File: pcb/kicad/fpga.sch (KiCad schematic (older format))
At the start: 15 parts, among them U4 XC3S400-PQ208

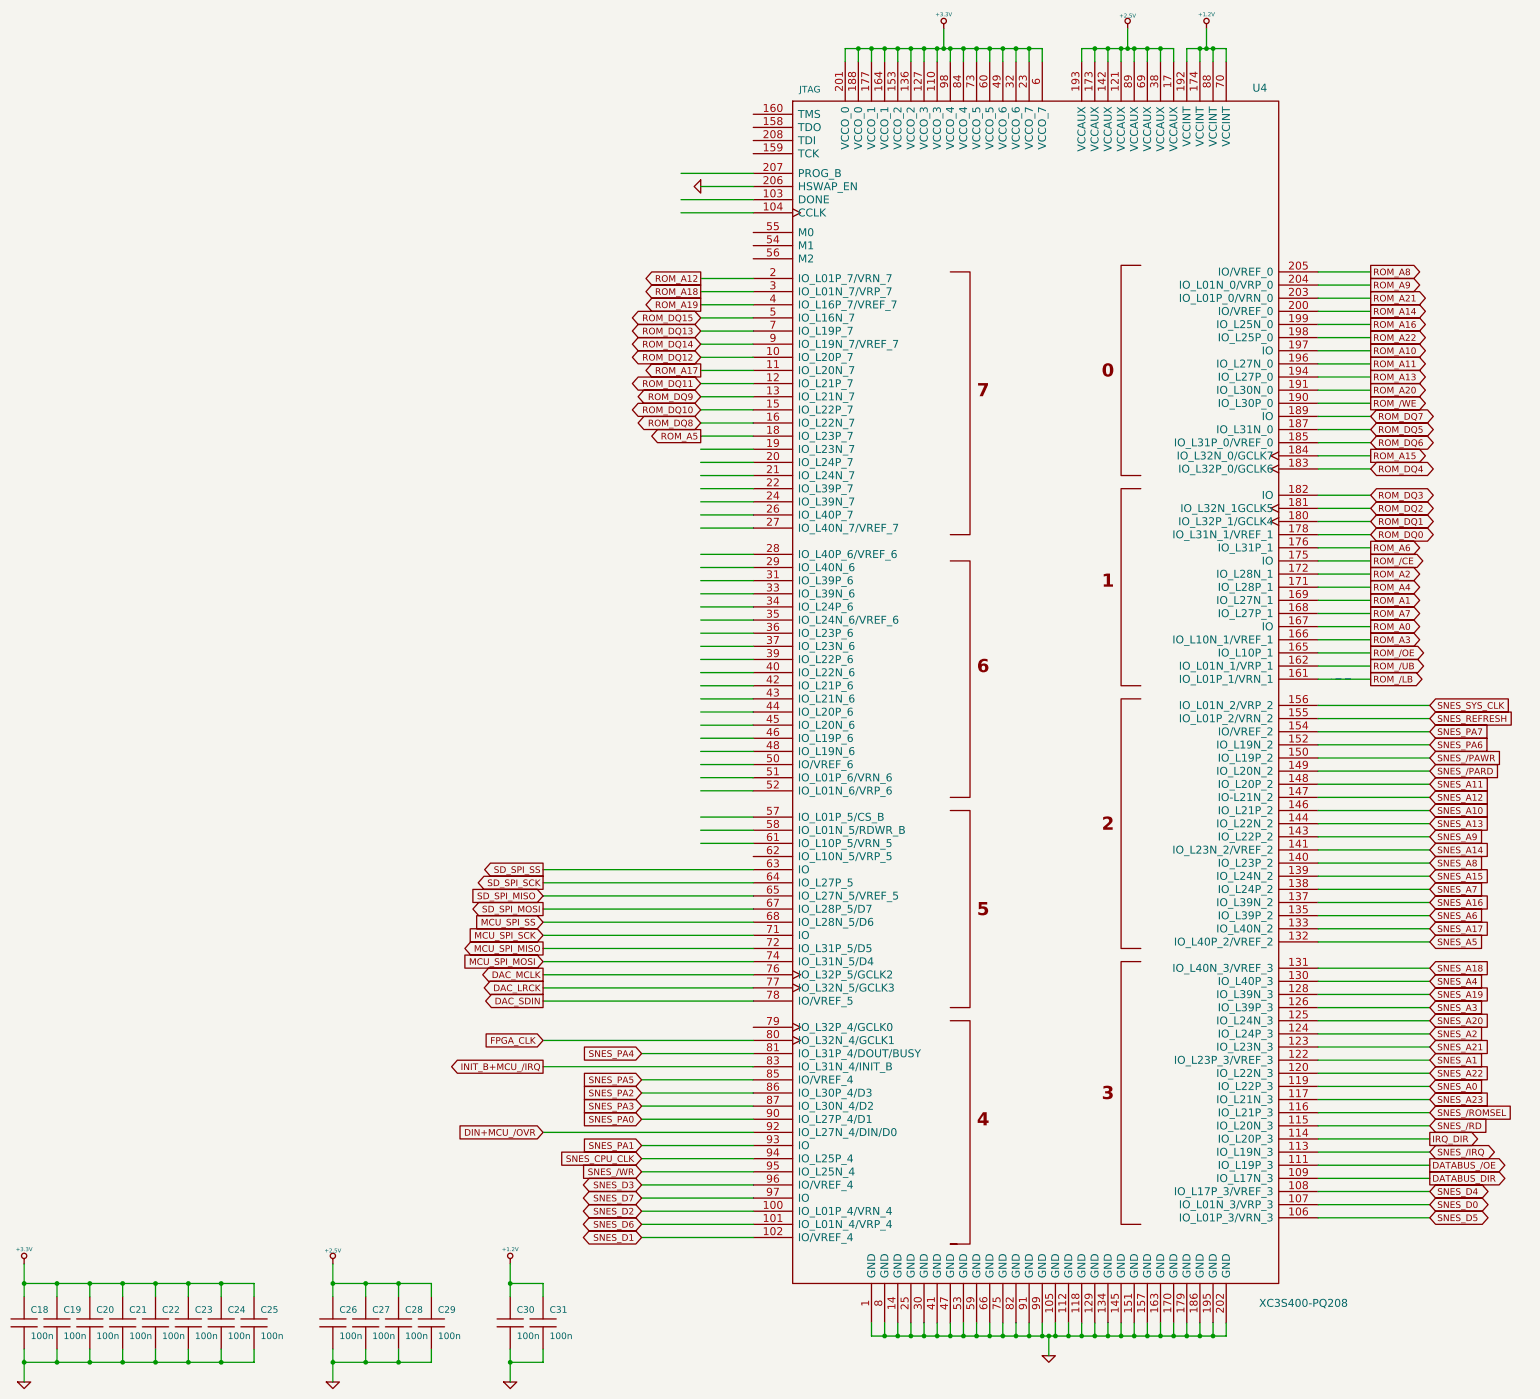
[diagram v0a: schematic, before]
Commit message: pcb wip
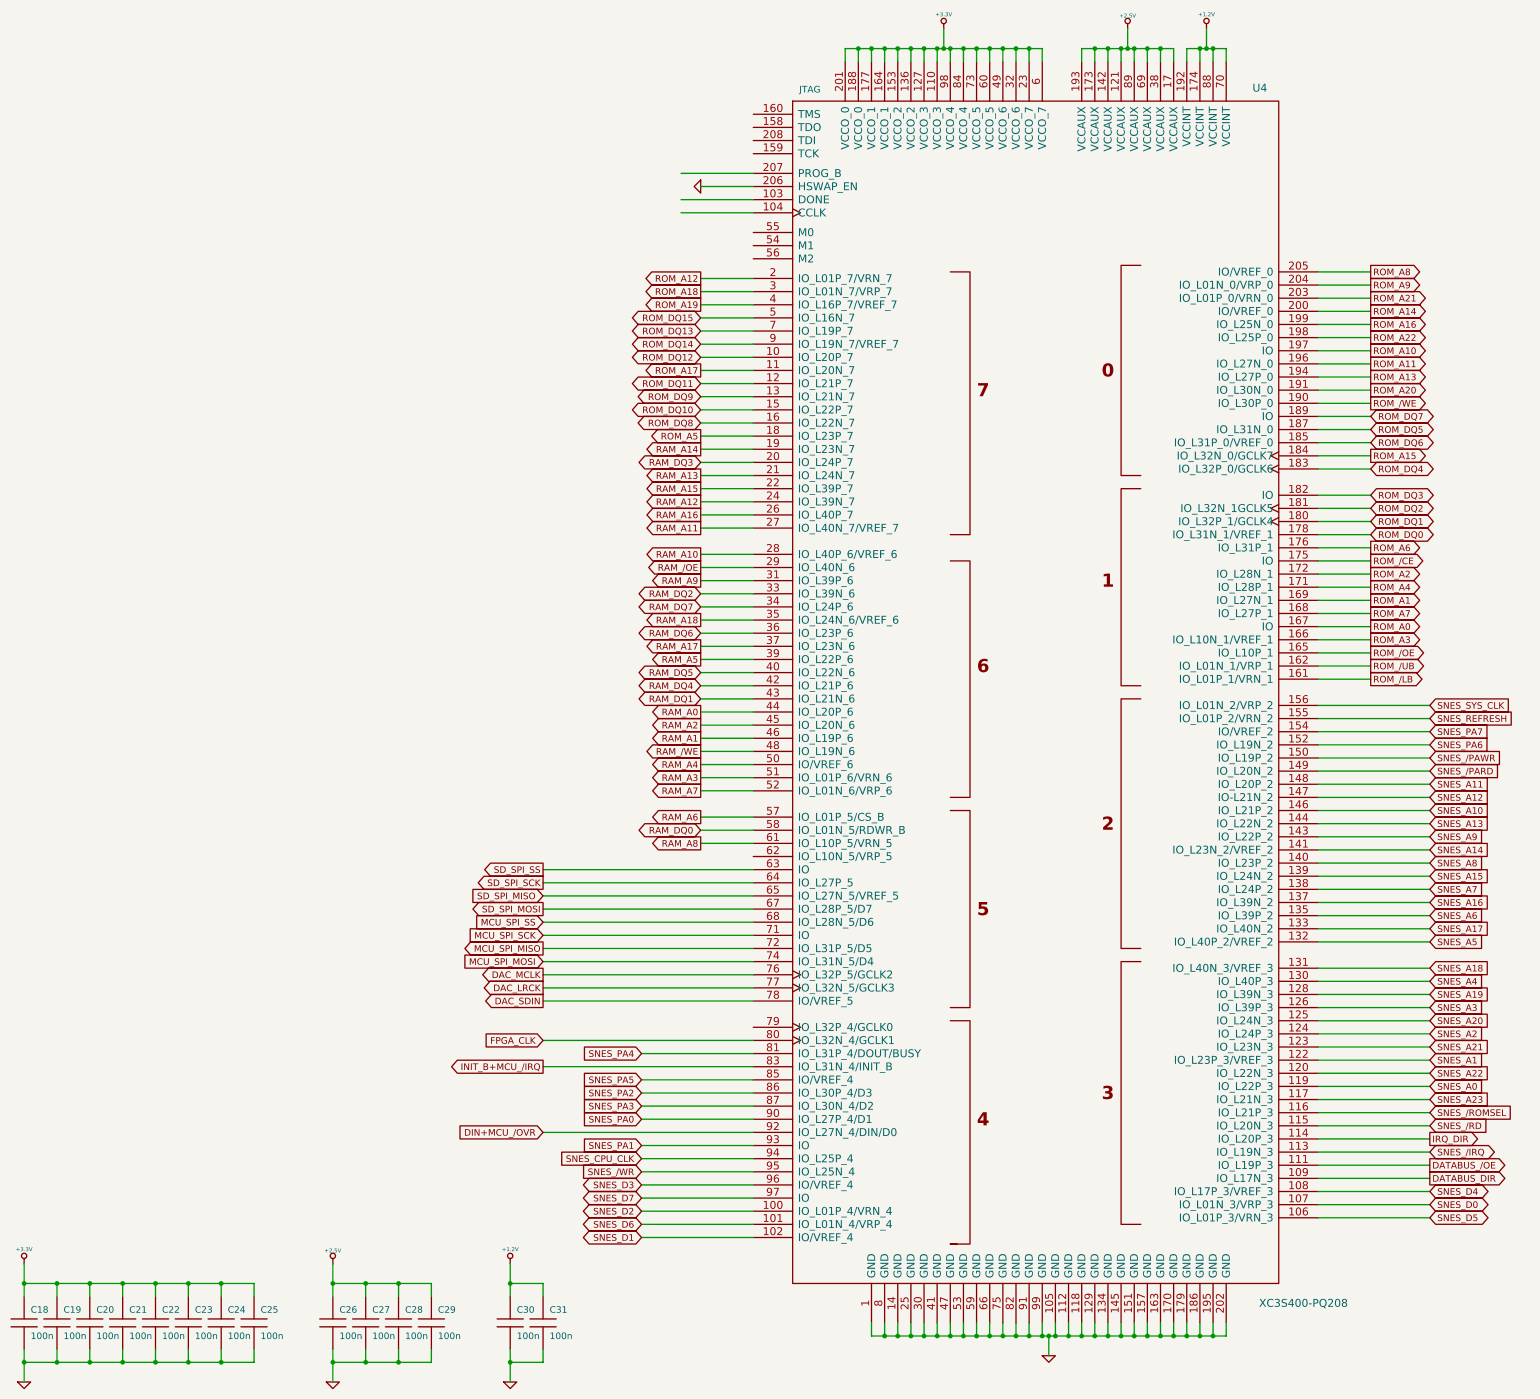
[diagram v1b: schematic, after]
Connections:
- net labels added: RAM_/OE, RAM_/WE, RAM_A0, RAM_A1, RAM_A10, RAM_A11, RAM_A12, RAM_A13, RAM_A14, RAM_A15, RAM_A16, RAM_A17, RAM_A18, RAM_A2, RAM_A3, RAM_A4, RAM_A5, RAM_A6, RAM_A7, RAM_A8, RAM_A9, RAM_DQ0, RAM_DQ1, RAM_DQ2, RAM_DQ3, RAM_DQ4, RAM_DQ5, RAM_DQ6, RAM_DQ7

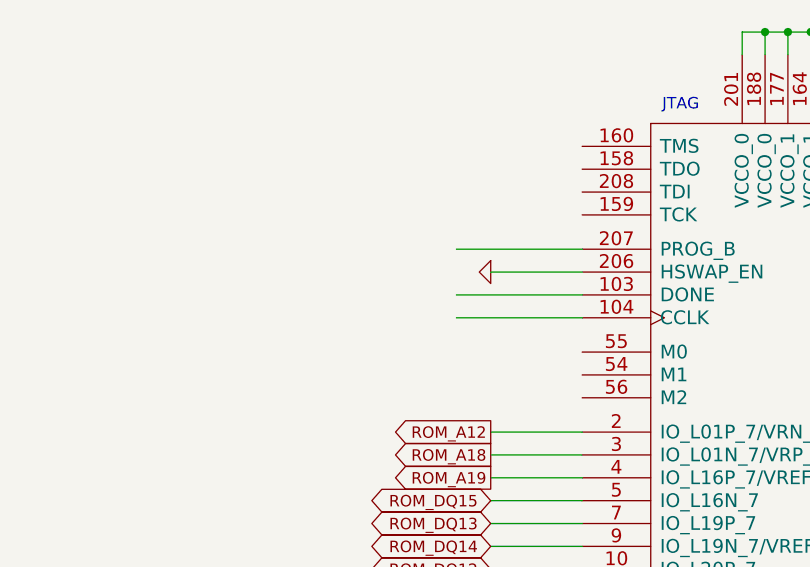
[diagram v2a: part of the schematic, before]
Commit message: pcb wip
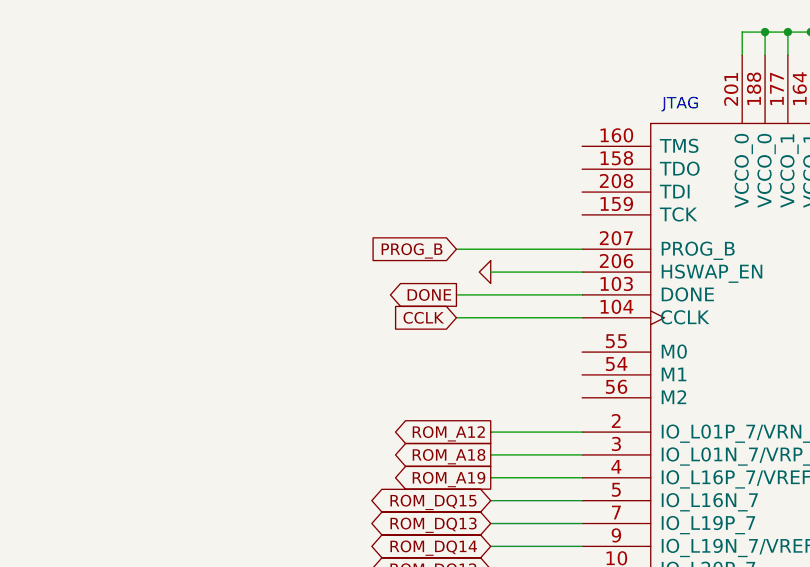
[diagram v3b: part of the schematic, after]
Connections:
- net DONE: now reaches U4.103 (DONE)
- net CCLK: now reaches U4.104 (CCLK)
- net PROG_B: now reaches U4.207 (PROG_B)
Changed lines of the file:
@@
-EESchema Schematic File Version 2  date Sat 15 May 2010 04:06:22 PM CEST
+EESchema Schematic File Version 2  date Sun 16 May 2010 01:08:34 AM CEST
 LIBS:power
 LIBS:device
@@
 Comment4 ""
 $EndDescr
+Text GLabel 5650 2200 0    50   Input ~ 0
+CCLK
+Text GLabel 5650 2100 0    50   Output ~ 0
+DONE
+Text GLabel 5650 1900 0    50   Input ~ 0
+PROG_B
 Wire Wire Line
 	10900 5750 10500 5750
@@
 SNES_SYS_CLK
 $Comp
-L GND #PWR080
+L GND #PWR084
 U 1 1 4BADE94E
 P 5800 2000
-F 0 "#PWR080" H 5800 2000 30  0001 C CNN
+F 0 "#PWR084" H 5800 2000 30  0001 C CNN
 F 1 "GND" H 5800 1930 30  0001 C CNN
 	1    5800 2000
@@
 $EndComp
 $Comp
-L GND #PWR081
+L GND #PWR085
 U 1 1 4BADE8CE
 P 8450 10900
-F 0 "#PWR081" H 8450 10900 30  0001 C CNN
+F 0 "#PWR085" H 8450 10900 30  0001 C CNN
 F 1 "GND" H 8450 10830 30  0001 C CNN
 	1    8450 10900
@@
 $EndComp
 $Comp
-L +1.2V #PWR082
+L +1.2V #PWR086
 U 1 1 4BADD09D
 P 4350 10200
-F 0 "#PWR082" H 4350 10340 20  0001 C CNN
+F 0 "#PWR086" H 4350 10340 20  0001 C CNN
 F 1 "+1.2V" H 4350 10310 30  0000 C CNN
 	1    4350 10200
@@
 $EndComp
 $Comp
-L +2.5V #PWR083
+L +2.5V #PWR087
 U 1 1 4BADD090
 P 3000 10200
-F 0 "#PWR083" H 3000 10150 20  0001 C CNN
+F 0 "#PWR087" H 3000 10150 20  0001 C CNN
 F 1 "+2.5V" H 3000 10300 30  0000 C CNN
 	1    3000 10200
@@
 $EndComp
 $Comp
-L GND #PWR084
+L GND #PWR088
 U 1 1 4BADD08B
 P 4350 11100
-F 0 "#PWR084" H 4350 11100 30  0001 C CNN
+F 0 "#PWR088" H 4350 11100 30  0001 C CNN
 F 1 "GND" H 4350 11030 30  0001 C CNN
 	1    4350 11100
@@
 $EndComp
 $Comp
-L GND #PWR085
+L GND #PWR089
 U 1 1 4BADD089
 P 3000 11100
-F 0 "#PWR085" H 3000 11100 30  0001 C CNN
+F 0 "#PWR089" H 3000 11100 30  0001 C CNN
 F 1 "GND" H 3000 11030 30  0001 C CNN
 	1    3000 11100
@@
 $EndComp
 $Comp
-L GND #PWR086
+L GND #PWR090
 U 1 1 4BADD072
 P 650 11100
-F 0 "#PWR086" H 650 11100 30  0001 C CNN
+F 0 "#PWR090" H 650 11100 30  0001 C CNN
 F 1 "GND" H 650 11030 30  0001 C CNN
 	1    650  11100
@@
 $EndComp
 $Comp
-L +3.3V #PWR087
+L +3.3V #PWR091
 U 1 1 4BADD05C
 P 650 10200
-F 0 "#PWR087" H 650 10160 30  0001 C CNN
+F 0 "#PWR091" H 650 10160 30  0001 C CNN
 F 1 "+3.3V" H 650 10310 30  0000 C CNN
 	1    650  10200
@@
 JTAG
 $Comp
-L +3.3V #PWR088
+L +3.3V #PWR092
 U 1 1 4BAD12D2
 P 7650 800
-F 0 "#PWR088" H 7650 760 30  0001 C CNN
+F 0 "#PWR092" H 7650 760 30  0001 C CNN
 F 1 "+3.3V" H 7650 910 30  0000 C CNN
 	1    7650 800
@@
 $EndComp
 $Comp
-L +2.5V #PWR089
+L +2.5V #PWR093
 U 1 1 4BAD12BE
 P 9050 800
-F 0 "#PWR089" H 9050 750 20  0001 C CNN
+F 0 "#PWR093" H 9050 750 20  0001 C CNN
 F 1 "+2.5V" H 9050 900 30  0000 C CNN
 	1    9050 800
@@
 $EndComp
 $Comp
-L +1.2V #PWR090
+L +1.2V #PWR094
 U 1 1 4BAD12B4
 P 9650 800
-F 0 "#PWR090" H 9650 940 20  0001 C CNN
+F 0 "#PWR094" H 9650 940 20  0001 C CNN
 F 1 "+1.2V" H 9650 910 30  0000 C CNN
 	1    9650 800
